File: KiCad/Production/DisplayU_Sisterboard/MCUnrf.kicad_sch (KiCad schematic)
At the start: 13 parts

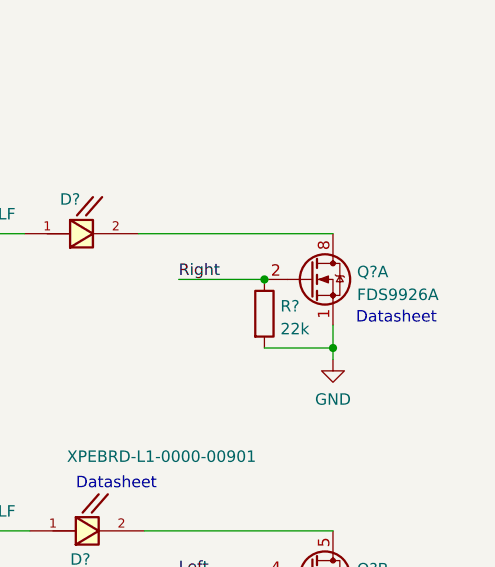
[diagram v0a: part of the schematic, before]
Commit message: Berekening/Metingen Verslag
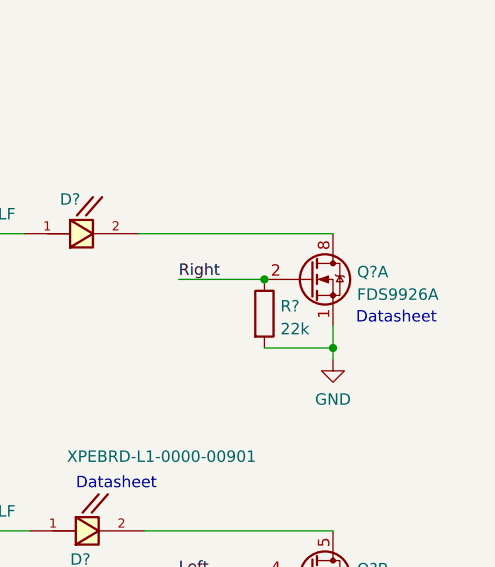
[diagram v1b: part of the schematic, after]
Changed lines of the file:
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@@
   (symbol (lib_id "Transistor_FET:FDS9926A") (at 254 77.47 0) (unit 1)
     (in_bom yes) (on_board yes) (dnp no) (fields_autoplaced)
-    (property "Reference" "Q?" (at 259.207 76.6353 0)
+    (property "Reference" "Q?" (at 259.207 76.6452 0)
       (effects (font (size 1.27 1.27)) (justify left))
     )
-    (property "Value" "FDS9926A" (at 259.207 79.1722 0)
+    (property "Value" "FDS9926A" (at 259.207 79.1504 0)
       (effects (font (size 1.27 1.27)) (justify left))
     )
